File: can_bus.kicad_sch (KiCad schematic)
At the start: 1 part, among them U8 MCP2562-E-SN

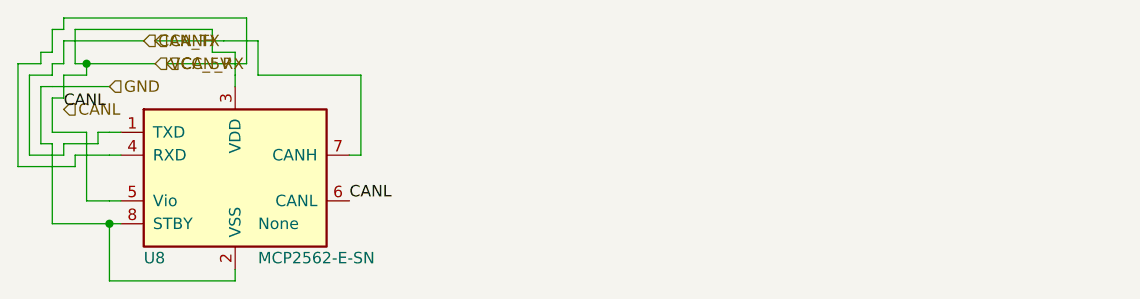
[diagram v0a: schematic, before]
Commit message: tests_fix
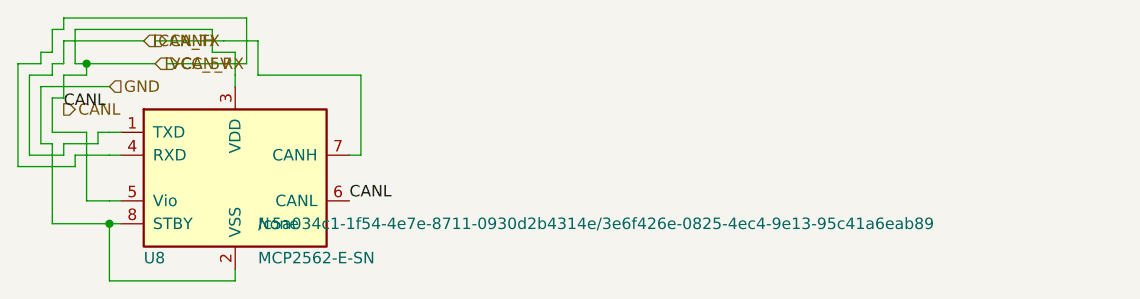
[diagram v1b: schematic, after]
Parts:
- U8: hierarchy_path (none) -> /c5a034c1-1f54-4e7e-8711-0930d2b4314e/3e6f426e-0825-4ec4-9e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
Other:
- title: (none) -> climate_control_niva_travel
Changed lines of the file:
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@@
 	(generator_version "9.0")
 	(paper "A4")
+	(title_block
+		(title "climate_control_niva_travel")
+	)
 	(symbol
 		(lib_id "Interface_CAN_LIN:MCP2562-E-SN")
@@
 			)
 		)
+		(property "hierarchy_path" "/c5a034c1-1f54-4e7e-8711-0930d2b4314e/3e6f426e-0825-4ec4-9e13-95c41a6eab89"
+			(at 38.1 29.2099 0)
+			(effects
+				(font
+					(size 1.27 1.27)
+				)
+				(justify left)
+			)
+		)
 		(pin "1"
 		)
@@
 		)
 		(instances
-			(project "Untitled"
-				(path "/deb6734f-8716-41b1-a872-d87713bf0c81"
+			(project "climate_control_niva_travel"
+				(path "/c5a034c1-1f54-4e7e-8711-0930d2b4314e/3e6f426e-0825-4ec4-9e13-95c41a6eab89"
 					(reference "U8")
 					(unit 1)
@@
 	)
 	(hierarchical_label "CAN_RX"
-		(shape input)
+		(shape output)
 		(at 27.94 11.43 0)
 		(effects
@@
 	)
 	(hierarchical_label "CANH"
-		(shape input)
+		(shape output)
 		(at 26.67 8.89 0)
 		(effects
@@
 	)
 	(hierarchical_label "CANL"
-		(shape input)
+		(shape output)
 		(at 16.51 16.51 0)
 		(effects
